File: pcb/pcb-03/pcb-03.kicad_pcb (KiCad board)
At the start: 2 copper layers, 50 x 30 mm, 12 parts, among them J1 S4B-PH-K-S HOST, J2 S8B-PH-K-S E-PAPER, U1 SC18IS606PWJ, U2 PCA9536DR

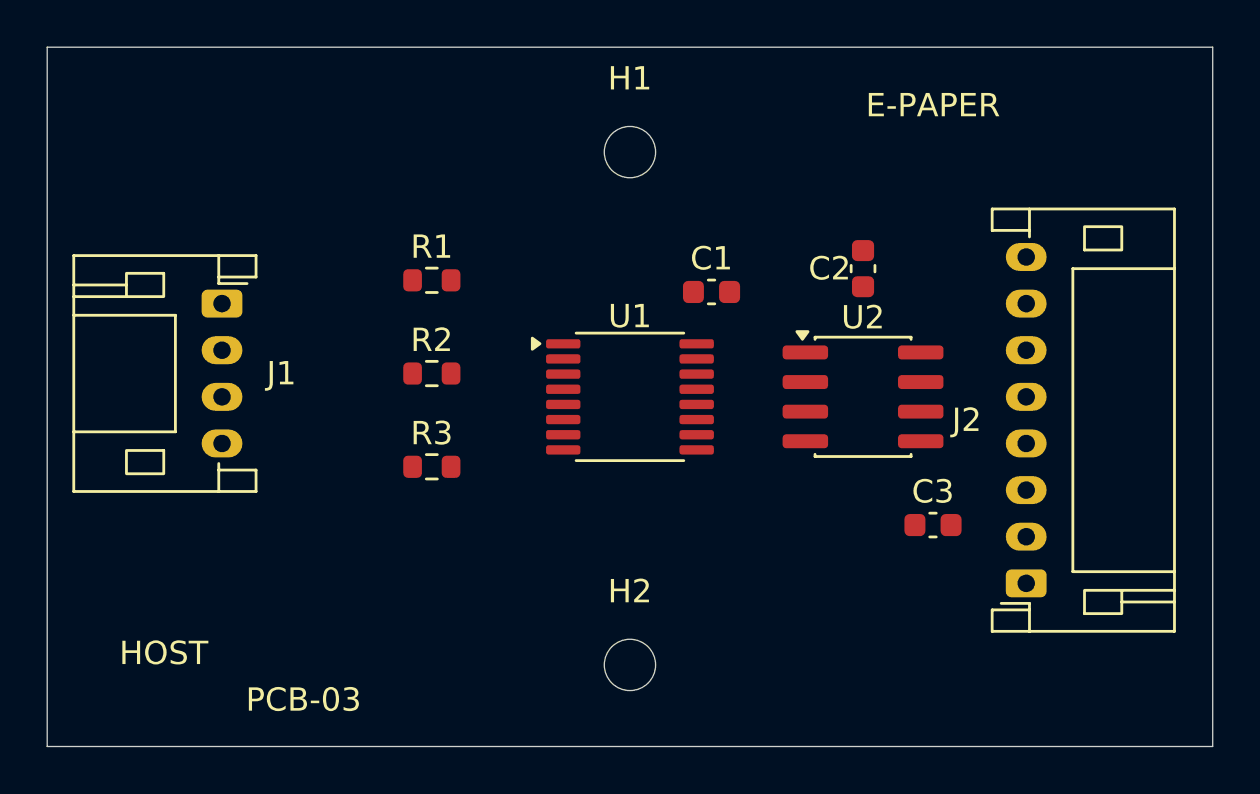
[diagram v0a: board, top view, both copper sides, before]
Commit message: Release PCB-03 bare-board fabrication package
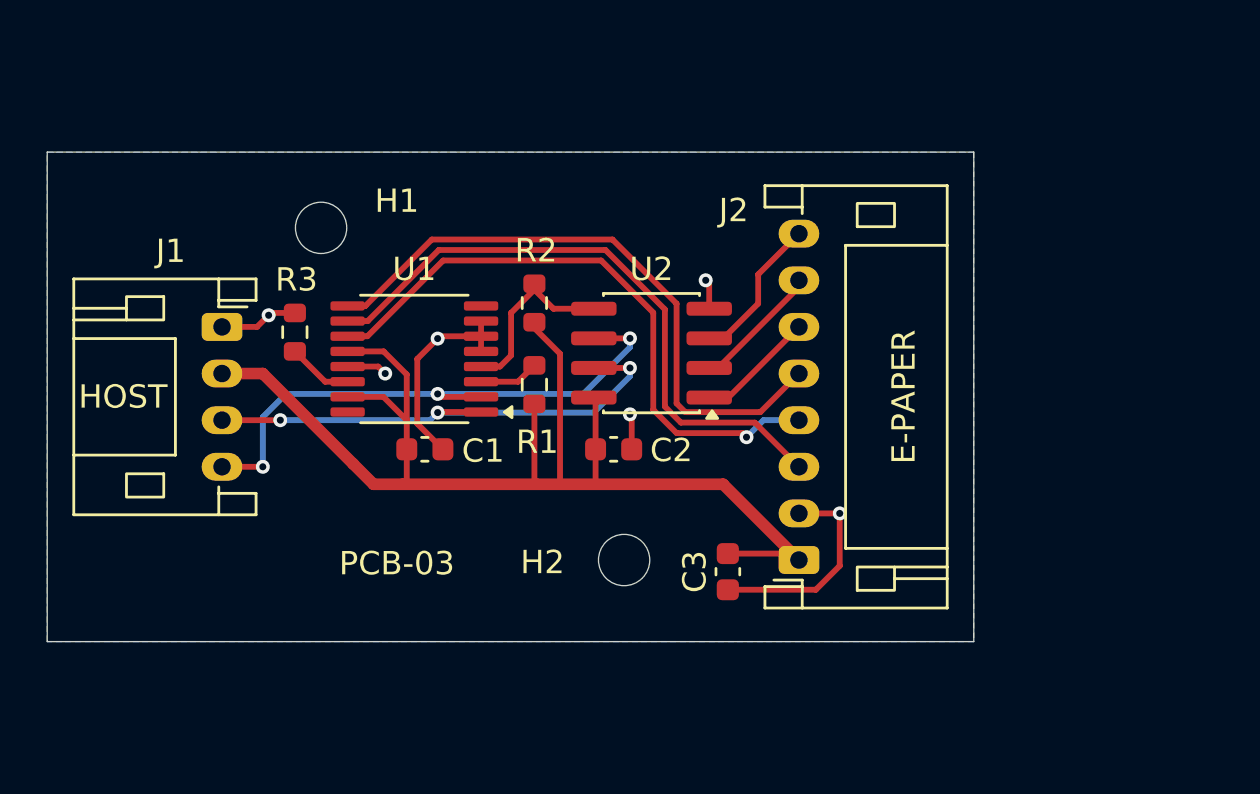
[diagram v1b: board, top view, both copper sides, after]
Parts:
- moved C1 14.0 mm to (66.2, 67.2)
- moved H1 13.6 mm to (61.8, 57.8)
- moved C2 13.2 mm to (74.3, 67.2), turned to 0 degrees
- moved J2 9.80 mm to (82.2, 72.0)
- moved U1 9.39 mm to (65.8, 63.4), turned to 180 degrees
- moved U2 9.27 mm to (75.9, 63.1), turned to 180 degrees
- moved C3 9.02 mm to (79.2, 72.5), turned to -90 degrees
- moved R3 8.24 mm to (60.6, 62.2), turned to 90 degrees
- moved R1 6.28 mm to (70.9, 64.5), turned to 90 degrees
- moved R2 5.34 mm to (70.9, 61.0), turned to 90 degrees
- moved H2 4.51 mm to (74.8, 72.0)
- moved J1 1.00 mm to (57.5, 62.0)
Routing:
- net /3V3: track 0.00 -> 56.3 mm
- net /EPD_DIN: track 0.00 -> 26.9 mm
- net /EPD_CS_N: track 0.00 -> 26.8 mm
- net /EPD_CLK: track 0.00 -> 26.6 mm, vias 0 -> 1
- net /AGND: track 0.00 -> 25.9 mm, vias 0 -> 6
- net /TEMP_SCL: track 0.00 -> 24.7 mm, vias 0 -> 3
- net /TEMP_SDA: track 0.00 -> 21.8 mm, vias 0 -> 3
- net /BRIDGE_RESET_N: track 0.00 -> 7.61 mm
- net /EPD_BUSY: track 0.00 -> 6.44 mm
- net /EPD_RESET_N: track 0.00 -> 5.58 mm
- net /EPD_DC: track 0.00 -> 5.11 mm
- net /CITO_PD: track 0.00 -> 2.80 mm
- net /BRIDGE_INT_N: track 0.00 -> 2.58 mm
- added copper zone on B.Cu, net /AGND
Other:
- board size 50 x 30 mm -> 39.8 x 21 mm
